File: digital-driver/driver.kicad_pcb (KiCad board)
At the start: 2 copper layers, 82.4 x 30.5 mm, 16 parts, among them J1 LDD-1500L, J2 Conn_01x02, J3 Barrel_Jack, J4 Conn_01x04, J5 Conn_01x04, J6 Barrel_Jack, J7 Conn_01x04, U1 ATtiny85-20PU

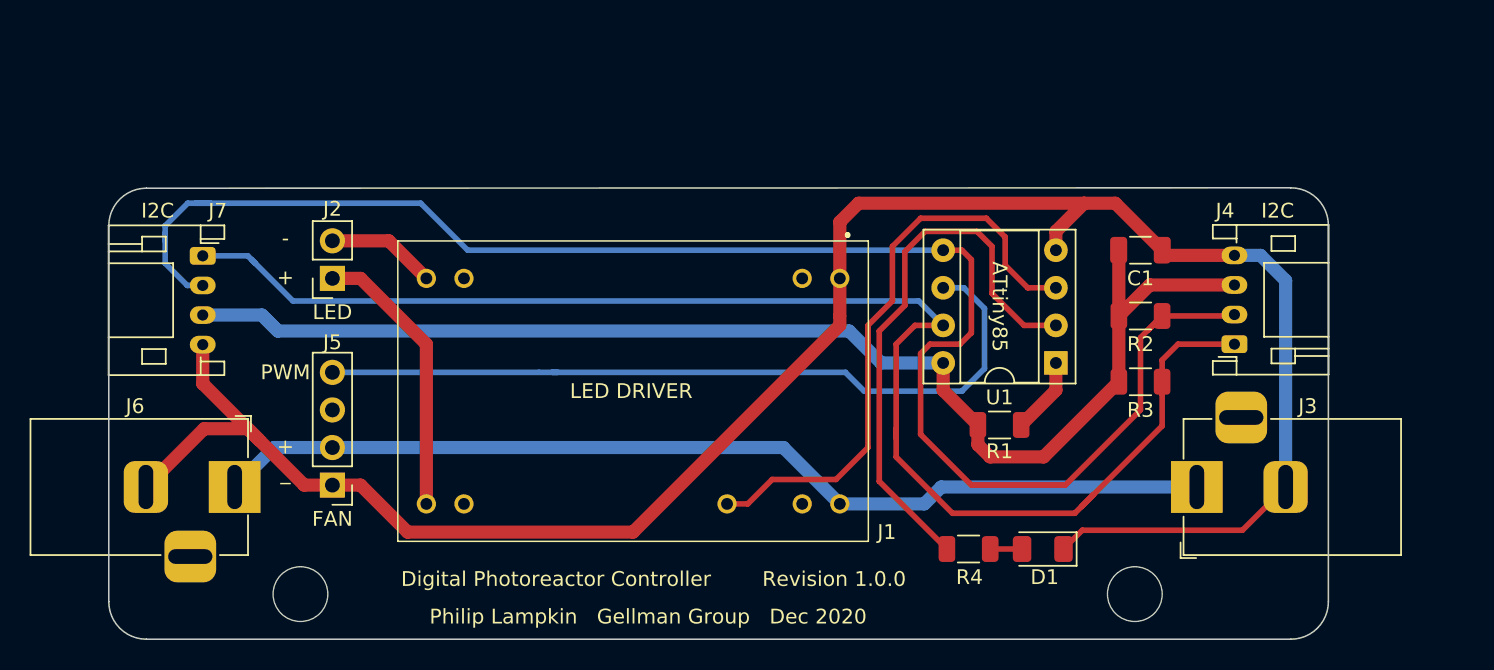
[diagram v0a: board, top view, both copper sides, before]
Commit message: digital driver prototype
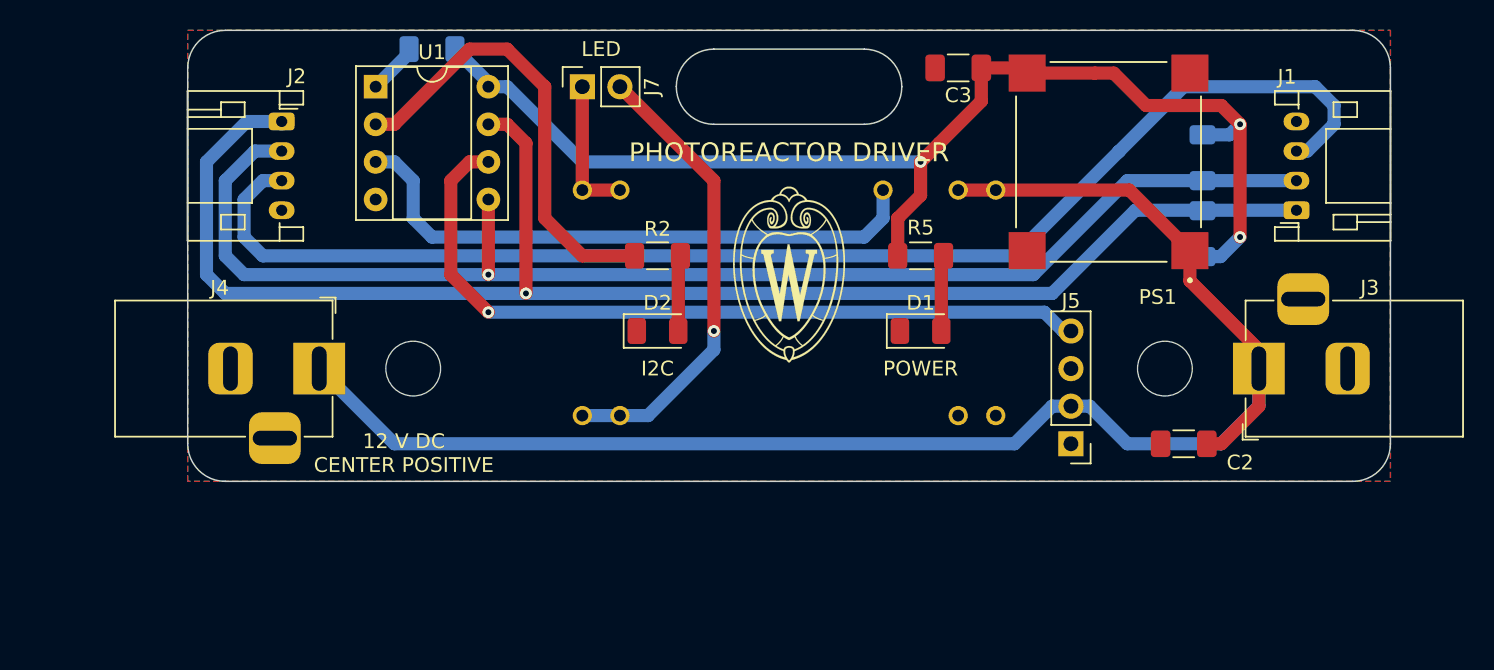
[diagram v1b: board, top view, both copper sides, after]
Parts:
- removed C1: 0.1uF, Capacitor_SMD:C_1206_3216Metric
- removed the J4 at (157.1, 99.9)
- removed the J7 at (87.4, 94.0)
- added C2: 10u, Capacitor_SMD:C_1206_3216Metric_Pad1.33x1.80mm_HandSolder, F.Cu at (153.7, 106.7)
- added C3: 22u, Capacitor_SMD:C_1206_3216Metric_Pad1.33x1.80mm_HandSolder, F.Cu at (138.4, 81.3)
- added D2: LED, LED_SMD:LED_1206_3216Metric, F.Cu at (118.1, 99.1)
- added G***: LOGO, footprints:logo, F.Cu at (127.0, 95.2)
- added J1: Conn_01x04, Connector_JST:JST_PH_S4B-PH-K_1x04_P2.00mm_Horizontal, F.Cu at (161.3, 90.9)
- added J2: Conn_01x04, Connector_JST:JST_PH_S4B-PH-K_1x04_P2.00mm_Horizontal, F.Cu at (92.7, 84.9)
- added PS1: VXO7805-500-M, footprints:CONV_VXO7805-500-M, F.Cu at (148.6, 87.6)
- added R5: 470, Resistor_SMD:R_1206_3216Metric_Pad1.30x1.75mm_HandSolder, F.Cu at (135.9, 94.0)
- J6: renamed from J1; moved to B.Cu
- R1: value 10K -> 4.7k; footprint Resistor_SMD:R_1206_3216Metric -> Resistor_SMD:R_1206_3216Metric_Pad1.30x1.75mm_HandSolder; moved to B.Cu
- R2: value 4.7K -> 470; footprint Resistor_SMD:R_1206_3216Metric -> Resistor_SMD:R_1206_3216Metric_Pad1.30x1.75mm_HandSolder
- R3: value 4.7K -> 10k; footprint Resistor_SMD:R_1206_3216Metric -> Resistor_SMD:R_1206_3216Metric_Pad1.30x1.75mm_HandSolder; moved to B.Cu
- R4: value 470 -> 4.7k; footprint Resistor_SMD:R_1206_3216Metric -> Resistor_SMD:R_1206_3216Metric_Pad1.30x1.75mm_HandSolder; moved to B.Cu
- moved R3 52.9 mm to (102.9, 80.0), turned to 180 degrees
- moved J5 50.0 mm to (146.1, 106.7)
- moved U1 49.6 mm to (99.1, 82.5), turned to 0 degrees
- moved R2 32.9 mm to (118.1, 94.0)
- moved R4 26.5 mm to (154.9, 92.5), turned to 90 degrees
- moved R1 22.7 mm to (154.9, 87.3), turned to 90 degrees
- moved J7 21.3 mm to (113.0, 82.5), turned to 90 degrees
- moved REF** 17.0 mm to (101.6, 101.6)
- moved D1 16.9 mm to (135.9, 99.1), turned to 0 degrees
- moved REF** 15.4 mm to (152.4, 101.6)
- moved J6 14.0 mm to (141.0, 104.8), turned to 90 degrees
- moved J4 9.83 mm to (95.2, 101.6)
- moved J3 9.03 mm to (158.8, 101.6)
- renumbered J6 to J4, J2 to J7
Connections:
- J6 pad 11: Net-(J1-Pad11) -> Net-(J6-Pad11)
- J6 pad 12: Net-(J1-Pad12) -> Net-(J6-Pad11)
- J6 pad 13: Net-(J1-Pad13) -> Net-(J6-Pad13)
- J6 pad 14: Net-(J1-Pad14) -> Net-(J6-Pad13)
- J6 pad 2: Net-(J1-Pad2) -> GND
- J6 pad 23: Net-(J1-Pad23) -> +12V
- J7 pad 1: Net-(J1-Pad13) -> Net-(J6-Pad13)
- J7 pad 2: Net-(J1-Pad12) -> Net-(J6-Pad11)
- R1 pad 1: +5V -> SDA
- R1 pad 2: Net-(R1-Pad2) -> +5V
- R2 pad 1: +5V -> INDICATOR
- R2 pad 2: SDA -> Net-(D2-Pad2)
- R3 pad 2: SCL -> Net-(R3-Pad2)
- R4 pad 1: Net-(D1-Pad2) -> +5V
- R4 pad 2: INDICATOR -> SCL
- U1 pad 1: Net-(R1-Pad2) -> Net-(R3-Pad2)
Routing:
- net GND: track 139.7 -> 0.00 mm
- net Net-(J1-Pad3): track 0.00 -> 89.7 mm
- net +12V: track 68.2 -> 106.9 mm
- net Net-(J6-Pad11): track 0.00 -> 31.1 mm, vias 0 -> 1
- net SDA: track 110.0 -> 90.3 mm, vias 0 -> 1
- net Net-(J1-Pad13): track 19.0 -> 0.00 mm
- net Net-(J6-Pad13): track 0.00 -> 9.52 mm
- net Net-(J1-Pad12): track 7.40 -> 0.00 mm
- net INDICATOR: track 38.0 -> 30.6 mm
- net +5V: track 88.6 -> 82.4 mm, vias 0 -> 3
- net Net-(R1-Pad2): track 5.16 -> 0.00 mm
- net Net-(D2-Pad2): track 0.00 -> 5.14 mm
- net SCL: track 99.5 -> 103.8 mm, vias 0 -> 1
- net Net-(R3-Pad2): track 0.00 -> 3.48 mm
- net Net-(D1-Pad2): track 2.16 -> 5.14 mm
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- added copper zone on B.Cu, net GND
- added copper zone on F.Cu, net GND
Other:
- board size 82.4 x 30.5 mm -> 81.3 x 30.5 mm
- net class Default: clearance 0.2 -> 0.381; trace_width 0.25 -> 0.889
- rule trace_clearance: 0.2 -> 0.381
- board text added: "12 V DC CENTER POSITIVE"
- board text added: "PHOTOREACTOR DRIVER"
- board text added: "POWER"
- board text added: "REVISION 1.0.0 JANUARY 2021"
- board text removed: "+"
- board text removed: "-"
- board text removed: "ATtiny85"
- board text removed: "Digital Photoreactor Controller"
- board text removed: "FAN"
- board text removed: "LED DRIVER"
- board text removed: "PWM"
- board text removed: "Philip Lampkin Gellman Group Dec 2020"
- board text removed: "Revision 1.0.0"
- board text removed: "_"
